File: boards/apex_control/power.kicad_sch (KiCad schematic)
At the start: 24 parts, among them U6 MIMXRT1171DVMAB, U7 TPS62086, U8 TPS62825, U9 LM66200, Y1 Crystal_GND24

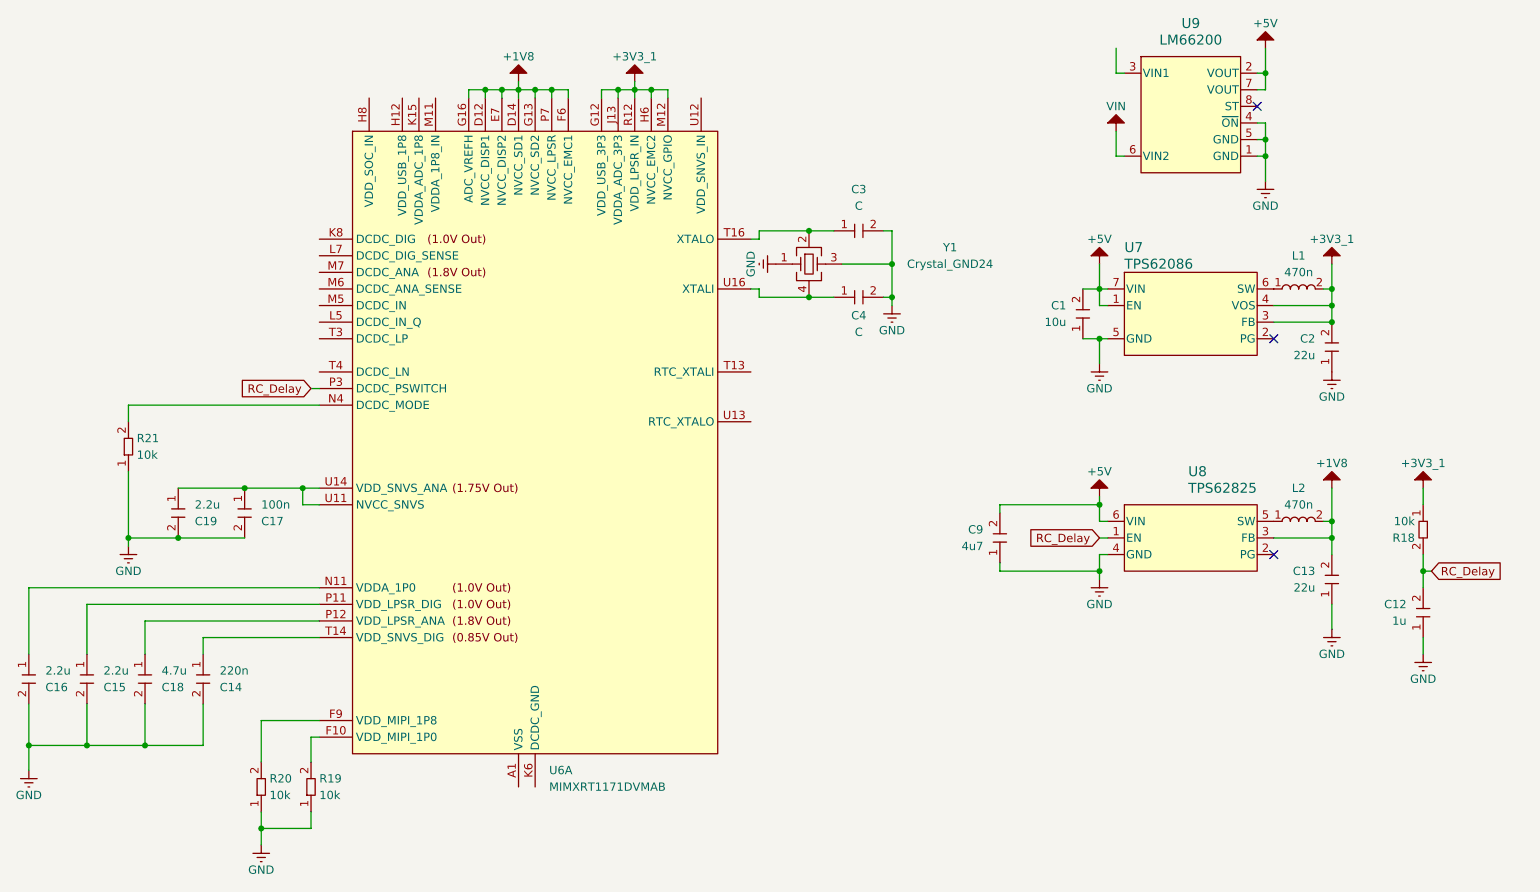
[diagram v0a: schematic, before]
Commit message: Worked on stuff
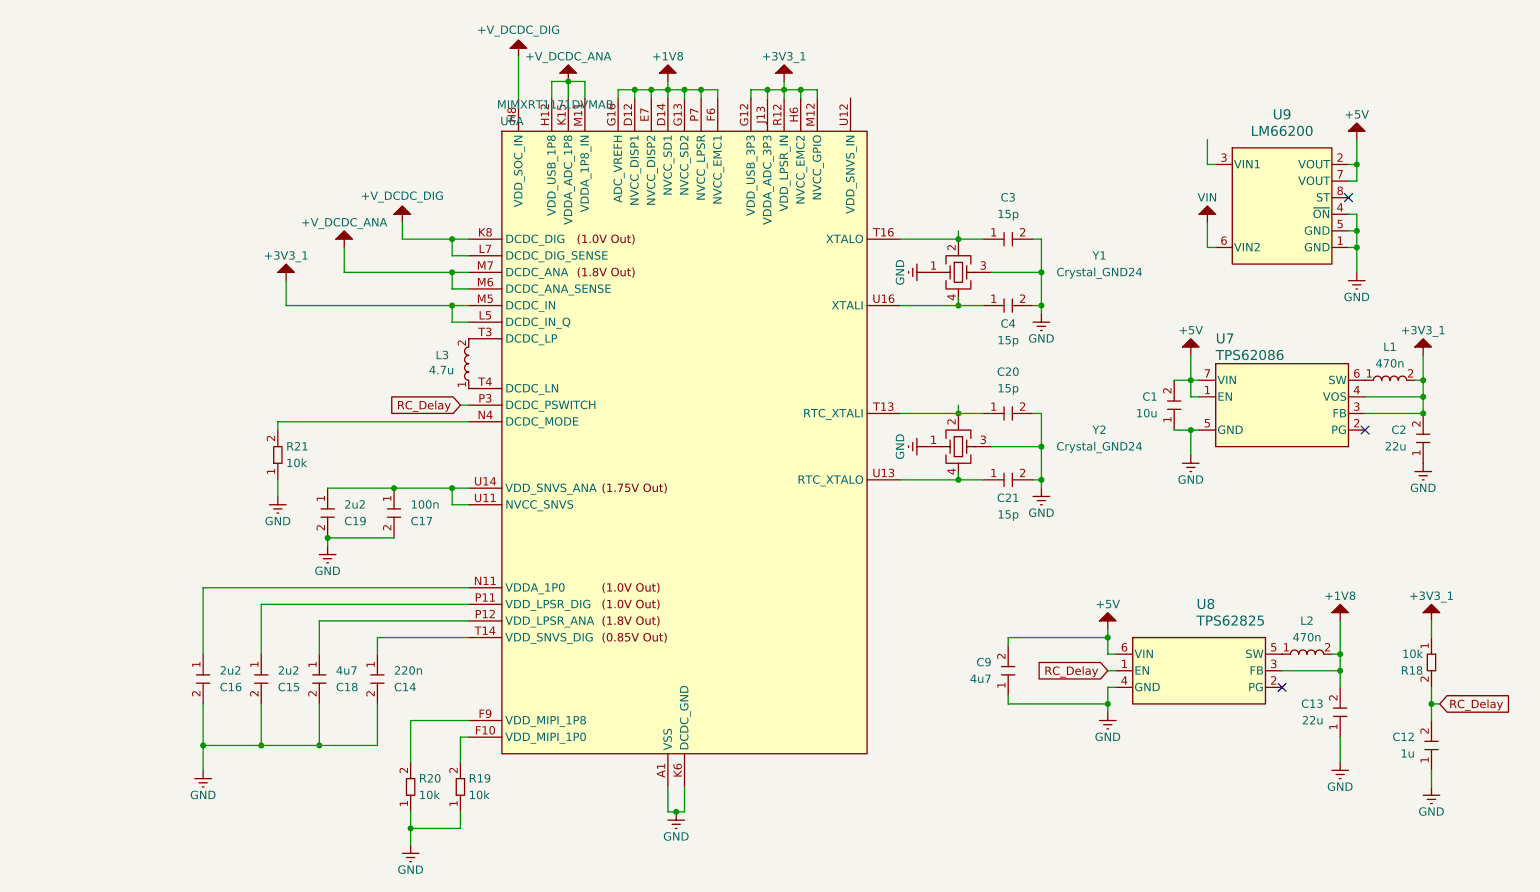
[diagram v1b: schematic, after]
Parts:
- added C20, C21: 15p, symbol APEX_Symbols:C
- added L3: 4.7u, symbol APEX_Symbols:L
- added Y2: Crystal_GND24, APEX_FOOTPRINTS:XTAL_3225, symbol APEX_Symbols:Crystal_GND24
- C15, C16, C19: value 2.2u -> 2u2
- C18: value 4.7u -> 4u7
- C3, C4: value C -> 15p
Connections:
- net +3V3_1: now also U6.L5 (DCDC_IN_Q), U6.M5 (DCDC_IN), U6.N5 (DCDC_IN)
- net GND: now also U6.A1 (VSS), U6.A17 (VSS), U6.B7 (VSS), U6.C10 (VSS), U6.C12 (VSS), U6.C14 (VSS), U6.C8 (VSS), U6.D4 (VSS), U6.F11 (VSS), U6.F12 (VSS), U6.F13 (VSS), U6.G10 (VSS), U6.G11 (VSS), U6.G15 (VSS), U6.G3 (VSS), U6.G7 (VSS), U6.G8 (VSS), U6.G9 (VSS), U6.H11 (VSS), U6.H7 (VSS), U6.J11 (VSS), U6.J7 (VSS), U6.K11 (VSS), U6.K6 (DCDC_GND), U6.K7 (DCDC_GND), U6.L10 (VSS), U6.L11 (VSS), U6.L15 (VSS), U6.L3 (VSS), U6.L6 (DCDC_GND), U6.P14 (VSS), U6.P4 (VSS), U6.R4 (VSS), U6.R7 (VSS), U6.T12 (VSS), U6.U1 (VSS), U6.U17 (VSS), C20.2, C21.2, Y2.1, Y2.3
- net +V_DCDC_DIG: now reaches U6.H10 (VDD_SOC_IN), U6.H8 (VDD_SOC_IN), U6.H9 (VDD_SOC_IN), U6.J10 (VDD_SOC_IN), U6.J8 (VDD_SOC_IN), U6.J9 (VDD_SOC_IN), U6.K10 (VDD_SOC_IN)
- net +V_DCDC_DIG: now also U6.K8 (DCDC_DIG), U6.K9 (DCDC_DIG), U6.L7 (DCDC_DIG_SENSE), U6.L8 (DCDC_DIG)
- net +V_DCDC_ANA: now reaches U6.H12 (VDD_USB_1P8)
- net +V_DCDC_ANA: now also U6.K15 (VDDA_ADC_1P8), U6.M11 (VDDA_1P8_IN), U6.M6 (DCDC_ANA_SENSE), U6.M7 (DCDC_ANA), U6.M8 (DCDC_ANA)
- net at U6.T13 (RTC_XTALI): now also C20.1, Y2.2 (GND)
- net at U6.T3 (DCDC_LP), U6.U3 (DCDC_LP): now also L3.2
- net at U6.T4 (DCDC_LN), U6.U4 (DCDC_LN): now also L3.1
- net at U6.U13 (RTC_XTALO): now also C21.1, Y2.4 (GND)
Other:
- moved on the sheet: C1, C12, C13, C14, C15, C16, C17, C18, C19, C2, C3, C4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
